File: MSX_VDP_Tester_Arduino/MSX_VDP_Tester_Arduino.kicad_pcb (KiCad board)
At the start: 2 copper layers, 83.8 x 61 mm, 22 parts, among them J1 VDP Under Test, J2 +5V In, J3 Power Passthrough, SW1 Test, U1 74LS595, U2 HDSP-7803, Y1 21.47MHz

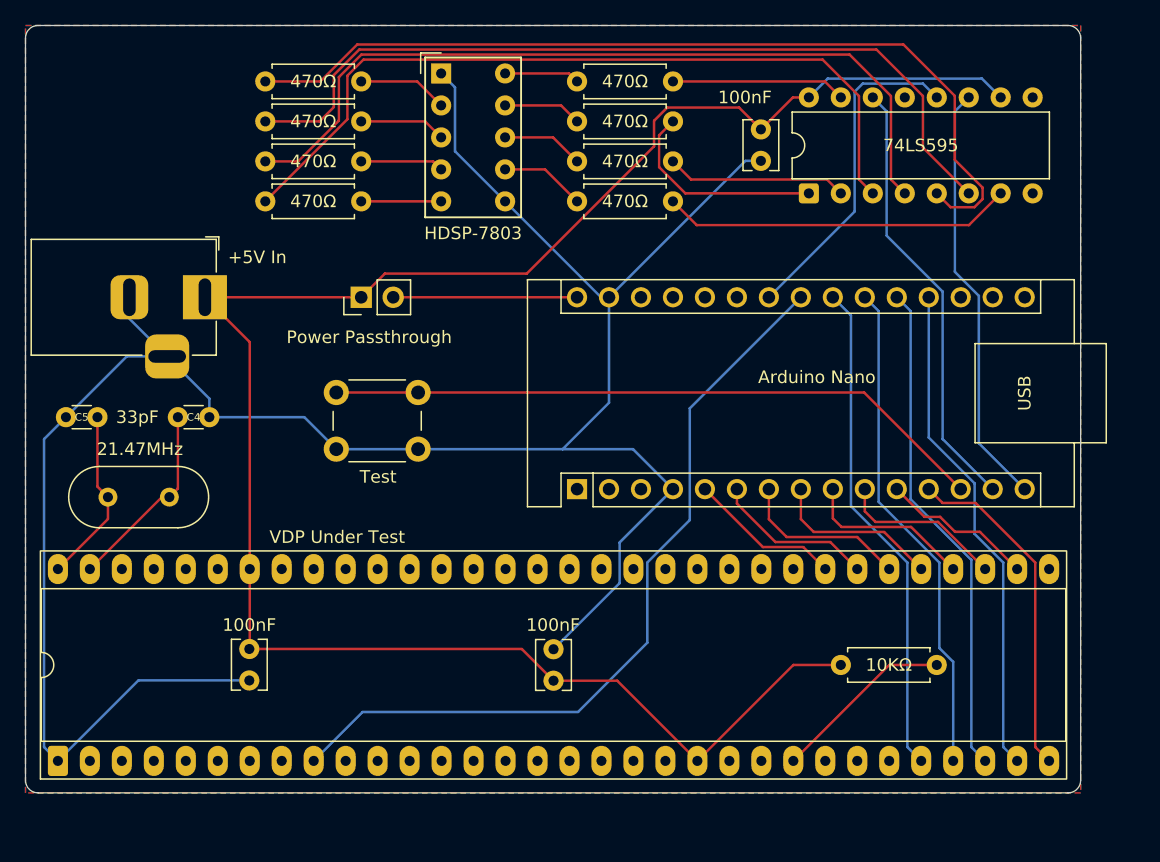
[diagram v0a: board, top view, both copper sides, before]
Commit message: Initial version for testing
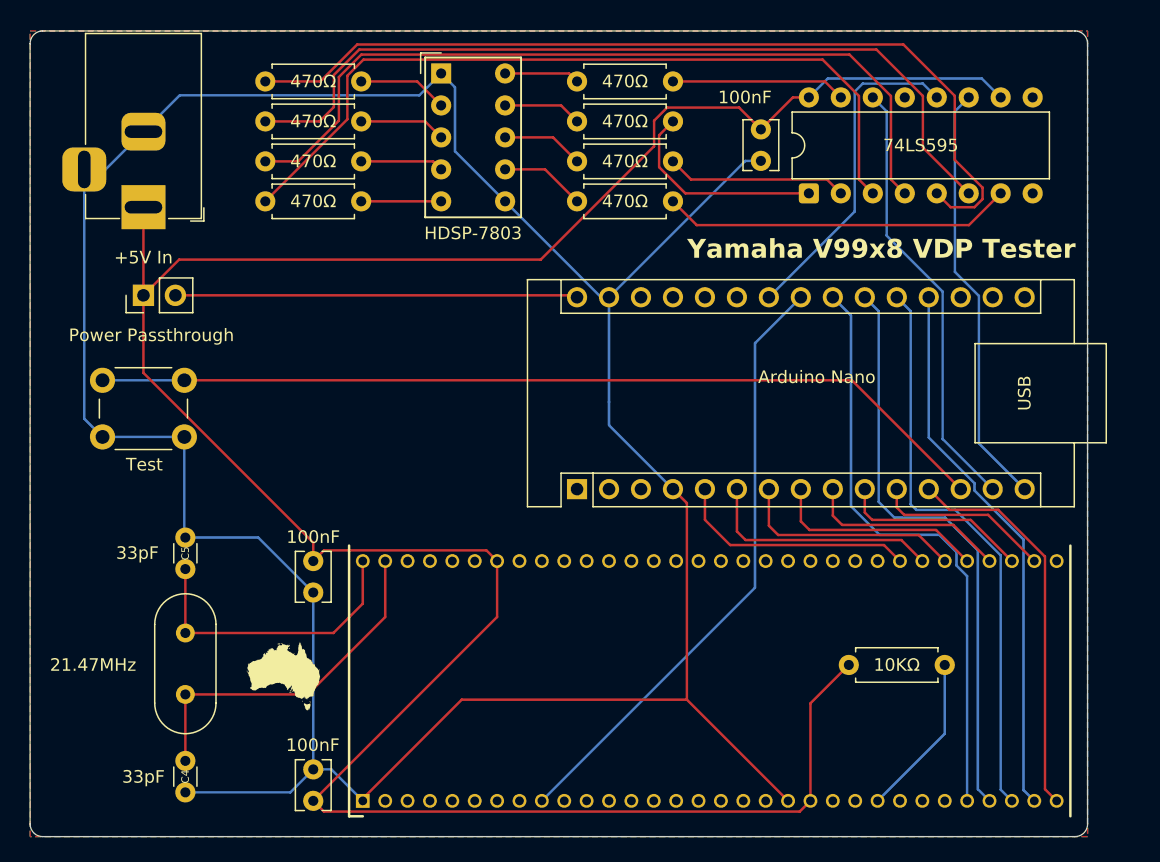
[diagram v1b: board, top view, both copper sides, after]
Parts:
- J1: footprint Package_DIP:DIP-64_W15.24mm_Socket_LongPads -> Clueless_Engineer:DIPS1905W50P178L5730H420Q64N
- moved C4 27.3 mm to (100.3, 134.0), turned to -90 degrees
- moved J1 24.4 mm to (114.4, 137.2)
- moved C1 21.3 mm to (110.5, 137.2)
- moved SW1 18.6 mm to (93.8, 103.8)
- moved J3 17.3 mm to (97.0, 97.0)
- moved C5 13.9 mm to (100.3, 118.7), turned to 90 degrees
- moved Y1 12.4 mm to (100.3, 123.8), turned to -90 degrees
- moved J2 8.66 mm to (97.0, 90.0), turned to -90 degrees
- moved C2 8.64 mm to (110.5, 118.1)
- moved R1 0.63 mm to (153.0, 126.4)
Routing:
- net /+5V: track 156.9 -> 204.8 mm
- net /GND: track 178.2 -> 225.2 mm
- net Net-(A1-D10): track 52.8 -> 71.8 mm
- net Net-(A1-VIN): track 14.6 -> 32.0 mm
- net /~{RESET}: track 62.9 -> 48.5 mm
- net /XTAL1: track 15.3 -> 28.1 mm
- net /XTAL2: track 14.1 -> 23.5 mm
- net /MODE1: track 39.7 -> 47.2 mm
- net /CD0: track 12.2 -> 19.3 mm
- net /MODE0: track 39.7 -> 46.5 mm
- net /CD1: track 12.9 -> 19.1 mm
- net /~{CSW}: track 39.7 -> 45.6 mm
- net /CD2: track 13.6 -> 18.0 mm
- net /CD7: track 27.1 -> 31.2 mm
- net /~{CSR}: track 39.7 -> 43.5 mm
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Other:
- board size 83.8 x 61 mm -> 84 x 64 mm
- board text added: "Brett Hallen, Jul 2026"
- board text added: "Yamaha V99x8 VDP Tester"
